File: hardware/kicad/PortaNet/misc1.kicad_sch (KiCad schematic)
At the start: 3 parts

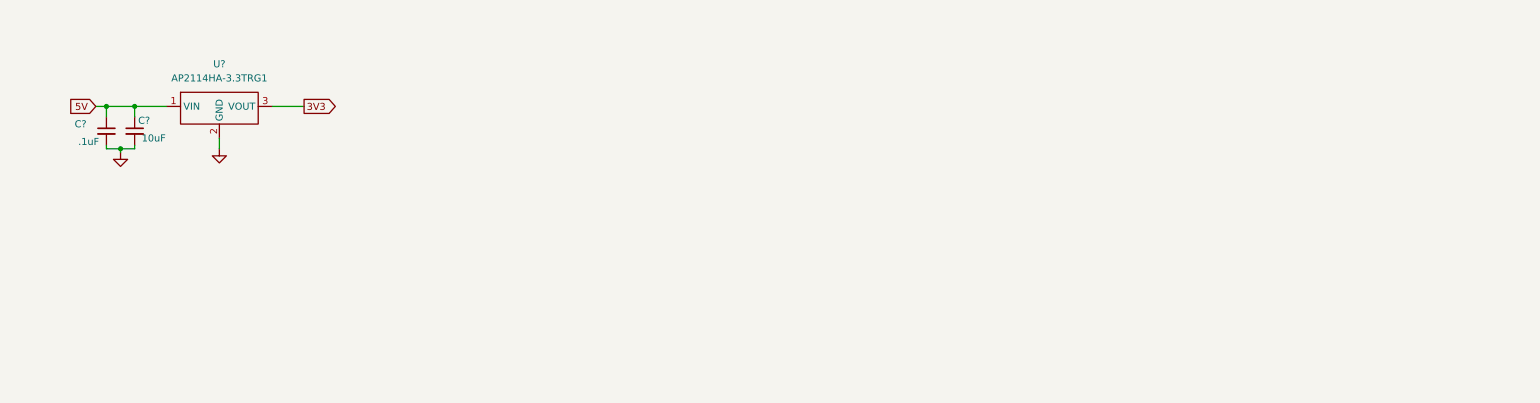
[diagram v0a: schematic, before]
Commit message: eod commit
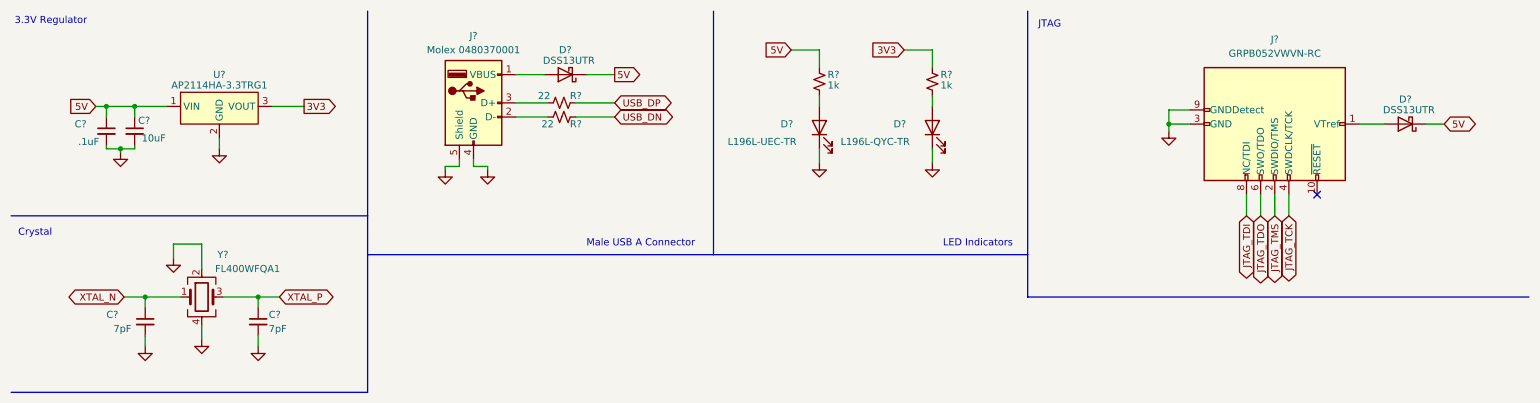
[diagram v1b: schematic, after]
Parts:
- added C? (x2): 7pF, Capacitor_SMD:C_0603_1608Metric, symbol Device:C_Small
- added D?: L196L-UEC-TR, LED_SMD:LED_0603_1608Metric, symbol Device:LED
- added D?: L196L-QYC-TR, LED_SMD:LED_0603_1608Metric, symbol Device:LED
- added D? (x2): DSS13UTR, Diode_SMD:D_SOD-123F, symbol Device:D_Schottky
- added J?: Molex 0480370001, JoesFootprints:Molex_0480370001, symbol Connector:USB_A
- added J?: GRPB052VWVN-RC, Connector_PinHeader_1.27mm:PinHeader_2x05_P1.27mm_Vertical, symbol Connector:Conn_ARM_JTAG_SWD_10
- added R? (x2): 1k, Resistor_SMD:R_0805_2012Metric, symbol Device:R_Small_US
- added R? (x2): 22, Resistor_SMD:R_0805_2012Metric, symbol Device:R_Small_US
- added Y?: FL400WFQA1, Crystal:Crystal_SMD_3225-4Pin_3.2x2.5mm, symbol Device:Crystal_GND24
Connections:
- net 3V3: now also R?.2
- net 5V: now also D?.1 (K), D?.1 (K), R?.2
- net GND: now also C?.2, C?.2, D?.1 (K), D?.1 (K), J?.3 (GND), J?.4 (GND), J?.5 (GND), J?.5 (Shield), J?.9 (GNDDetect), Y?.2, Y?.4
- new net: D?.2 (A), R?.1 (x2)
- new net: D?.2 (A), J?.1 (VBUS)
- new net: J?.2 (D-), R?.1
- new net: J?.3 (D+), R?.1
- new net: D?.2 (A), J?.1 (VTref)
- new net JTAG_TCK: J?.4 (SWDCLK/TCK)
- new net JTAG_TDI: J?.8 (NC/TDI)
- new net JTAG_TDO: J?.6 (SWO/TDO)
- new net JTAG_TMS: J?.2 (SWDIO/TMS)
- new net USB_DN: R?.2
- new net USB_DP: R?.2
- new net XTAL_N: C?.1, Y?.1
- new net XTAL_P: C?.1, Y?.3
- no-connect marks 0 -> 1
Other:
- note added: "3.3V Regulator"
- note added: "Crystal"
- note added: "JTAG"
- note added: "LED Indicators"
- note added: "Male USB A Connector"
